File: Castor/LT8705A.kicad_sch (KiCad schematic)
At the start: 45 parts, among them J1 IPS1-105-01-L-D, J6 IPS1-105-01-L-D, Q3 SQJ850EP, Q4 SQJ886EP, Q5 SQJ486EP, Q6 SQJ410EP, U8 TPS16851VMAR, U9 LT8705AxFE

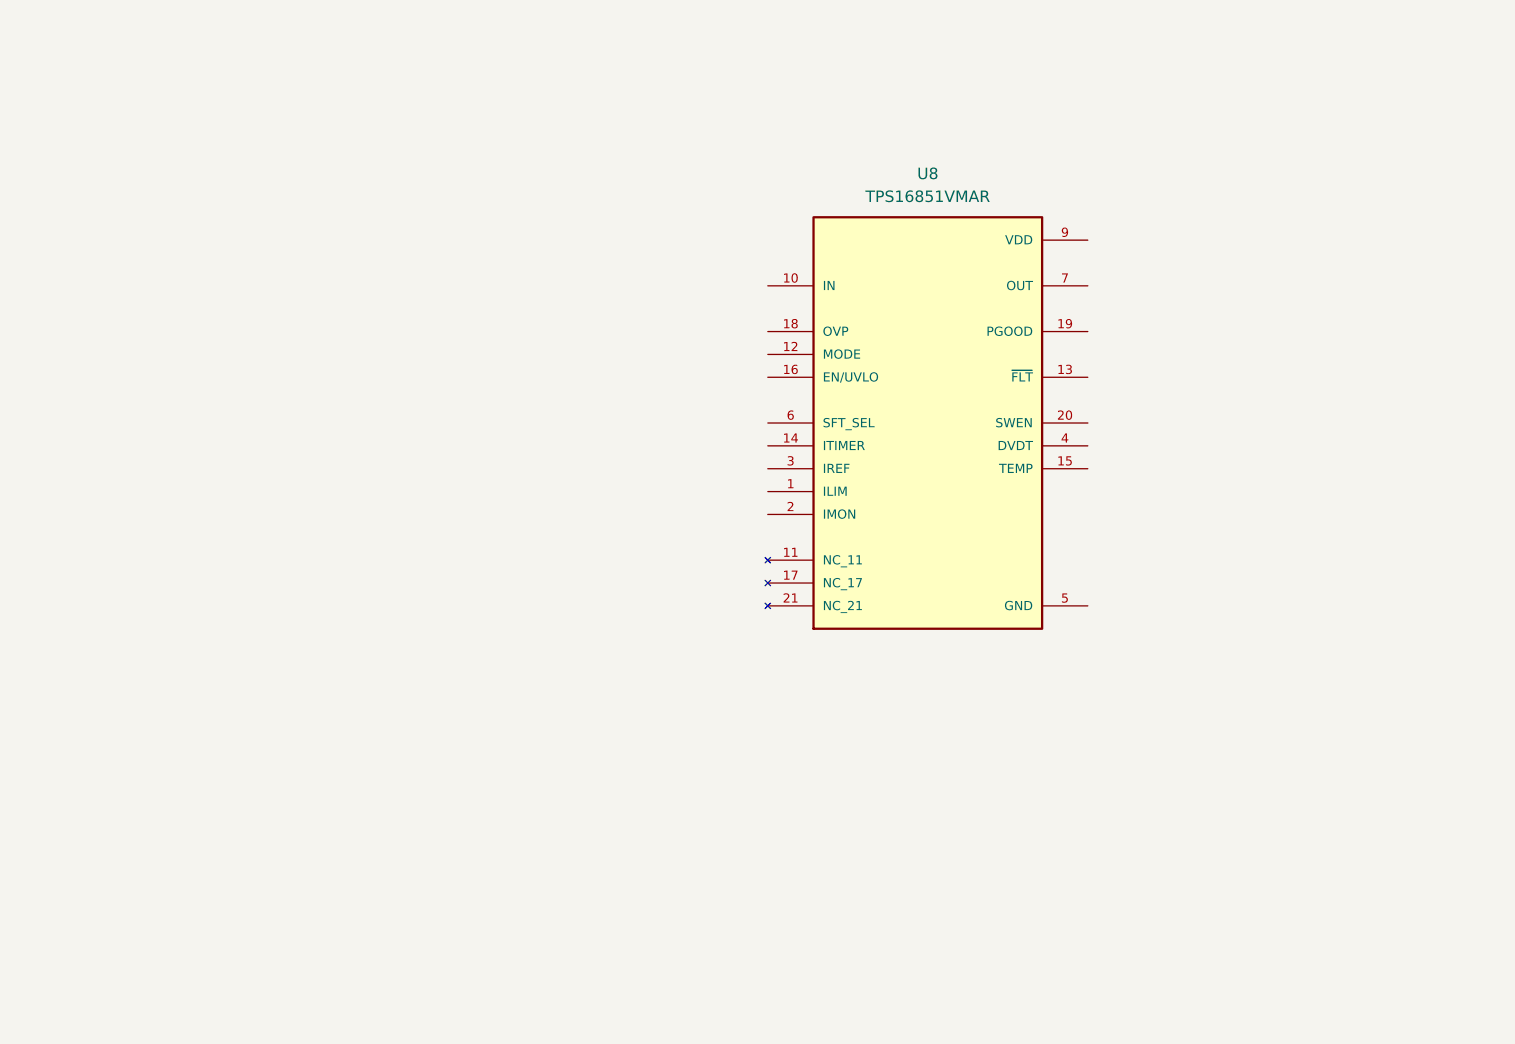
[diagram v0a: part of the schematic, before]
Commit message: castor
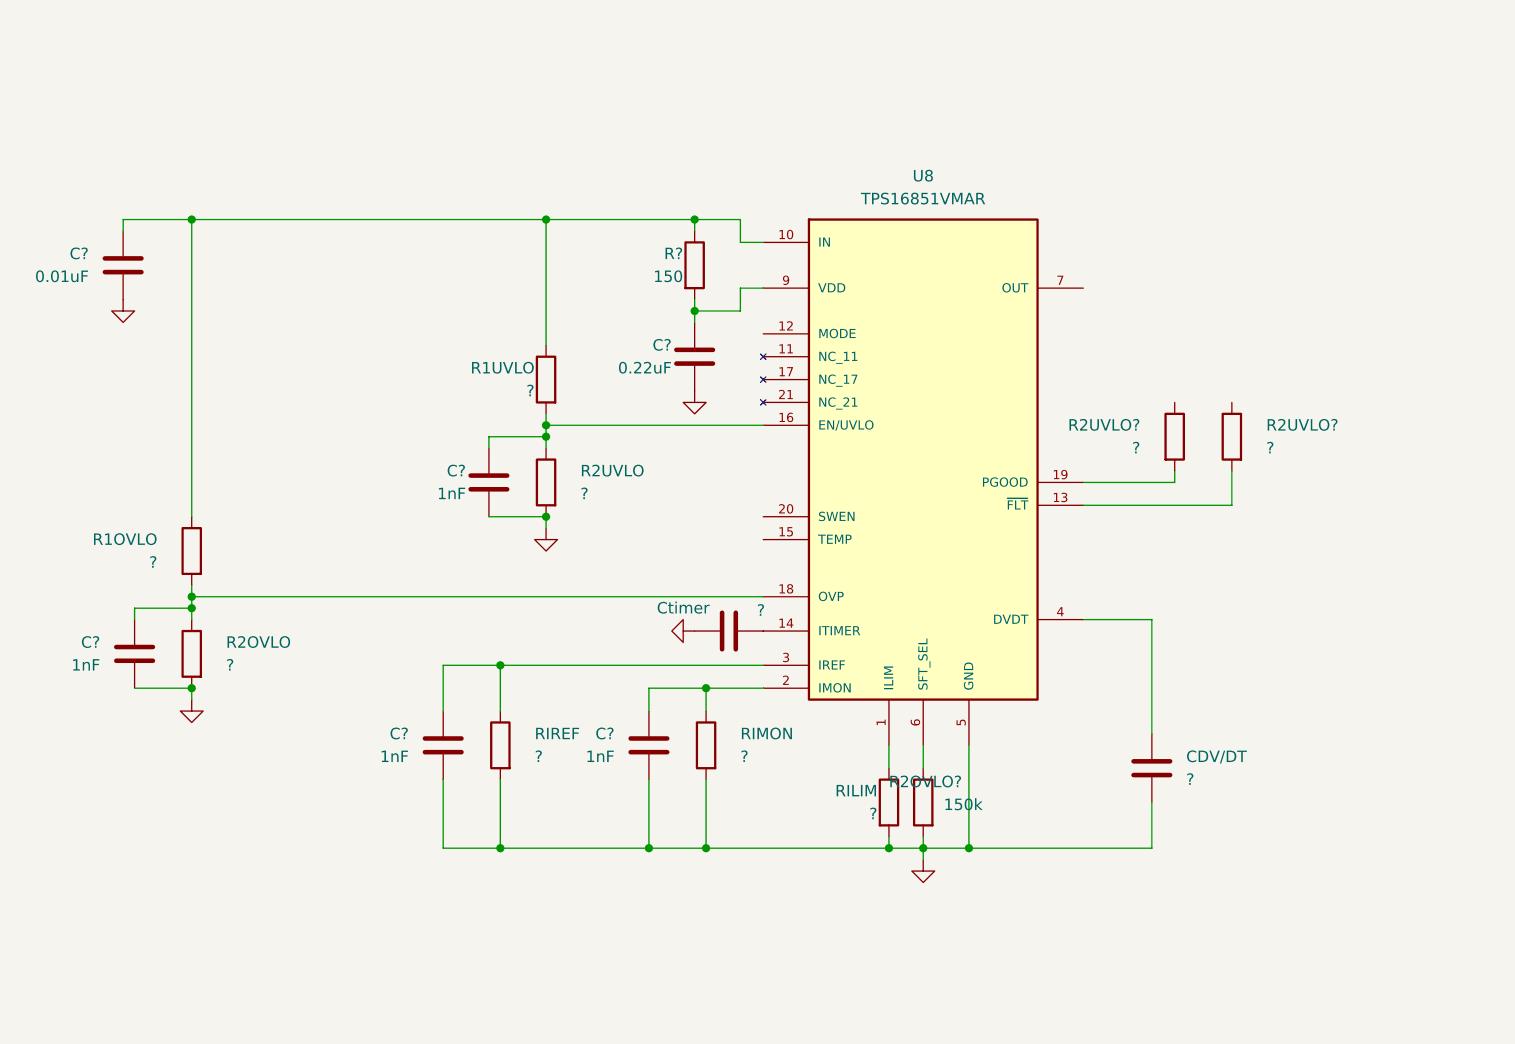
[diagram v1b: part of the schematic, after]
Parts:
- added C? (x4): 1nF, Capacitor_SMD:C_1210_3225Metric, symbol Device:C
- added C?: 0.22uF, Capacitor_SMD:C_1210_3225Metric, symbol Device:C
- added C?: 0.01uF, Capacitor_SMD:C_1210_3225Metric, symbol Device:C
- added CDV/DT, Ctimer: ?, Capacitor_SMD:C_1210_3225Metric, symbol Device:C
- added R1OVLO, R1UVLO, R2OVLO, R2UVLO, R2UVLO? (x2), RILIM, RIMON, RIREF: ?, Resistor_SMD:R_0603_1608Metric, symbol Device:R
- added R2OVLO?: 150k, Resistor_SMD:R_0603_1608Metric, symbol Device:R
- added R?: 150, Resistor_SMD:R_0603_1608Metric, symbol Device:R
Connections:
- net GND: now also U8.5 (GND), C?.1, C?.1, C?.1, C?.1, C?.1, C?.1, CDV/DT.1, Ctimer.2, R2OVLO.2, R2OVLO?.2, R2UVLO.2, RILIM.2, RIMON.2, RIREF.2
- net IN: now also C?.2, R1OVLO.1, R1UVLO.1, R?.1
- net at U8.1 (ILIM): now also RILIM.1
- net at U8.13 (~{FLT}): now also R2UVLO?.2
- net at U8.14 (ITIMER): now also Ctimer.1
- net at U8.16 (EN/UVLO): now also C?.2, R1UVLO.2, R2UVLO.1
- net at U8.18 (OVP): now also C?.2, R1OVLO.2, R2OVLO.1
- net at U8.19 (PGOOD): now also R2UVLO?.2
- net at U8.2 (IMON): now also C?.2, RIMON.1
- net at U8.3 (IREF): now also C?.2, RIREF.1
- net at U8.4 (DVDT): now also CDV/DT.2
- net at U8.6 (SFT_SEL): now also R2OVLO?.1
- net at U8.9 (VDD): now also C?.2, R?.2
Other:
- moved on the sheet: U8
